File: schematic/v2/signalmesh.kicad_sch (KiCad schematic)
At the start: 164 parts, among them J1 FPGA I/O, J10 INA219_CONFIG, J11 INA219_CONFIG, J12 AAM_DBG, J13 UUM_DBG, J14 ACM_DBG, J15 INA219_CONFIG, J16 DSM_DBG, J17 LCD_display, J18 LCD_display, J19 AudioJack3, J2 FPGA I/O, J20 USB3_A, J21 USB_A, J23 USB_A, J3 LCD_display, J4 TDM_DBG, J5 INA219_CONFIG, J6 INA219_CONFIG, J7 INA219_CONFIG, J8 FPGA I/O, J9 FPGA I/O, U1 NUCLEO-H753ZI, U10 INA219AxD, U11 INA219AxD, U12 INA219AxD, U13 INA219AxD, U14 W25Q128JVS, U15 AP2112K-3.3, U16 74HC4050D, U17 NUCLEO-H753ZI, U18 HDSP-7503, U19 HDSP-7503, U2 HDSP-7503, U20 INA219AxD, U21 74HC4050D, U22 AP2112K-3.3, U23 W25Q128JVS, U24 74HC4050D, U25 AP2112K-3.3, U26 W25Q128JVS, U27 MCP2551-I-P, U28 74LVC1G3157, U29 MCP2551-I-P, U3 NUCLEO-F303RE, U30 MCP2551-I-P, U31 MCP2551-I-P, U32 CH340G, U4 YAAJ_BluePill_Part_Like, U5 24LC256-I_SN, U6 BME280, U7 INA219AxD, U8 24LC256-I_SN, U9 NUCLEO-F446RE, Y1 Crystal

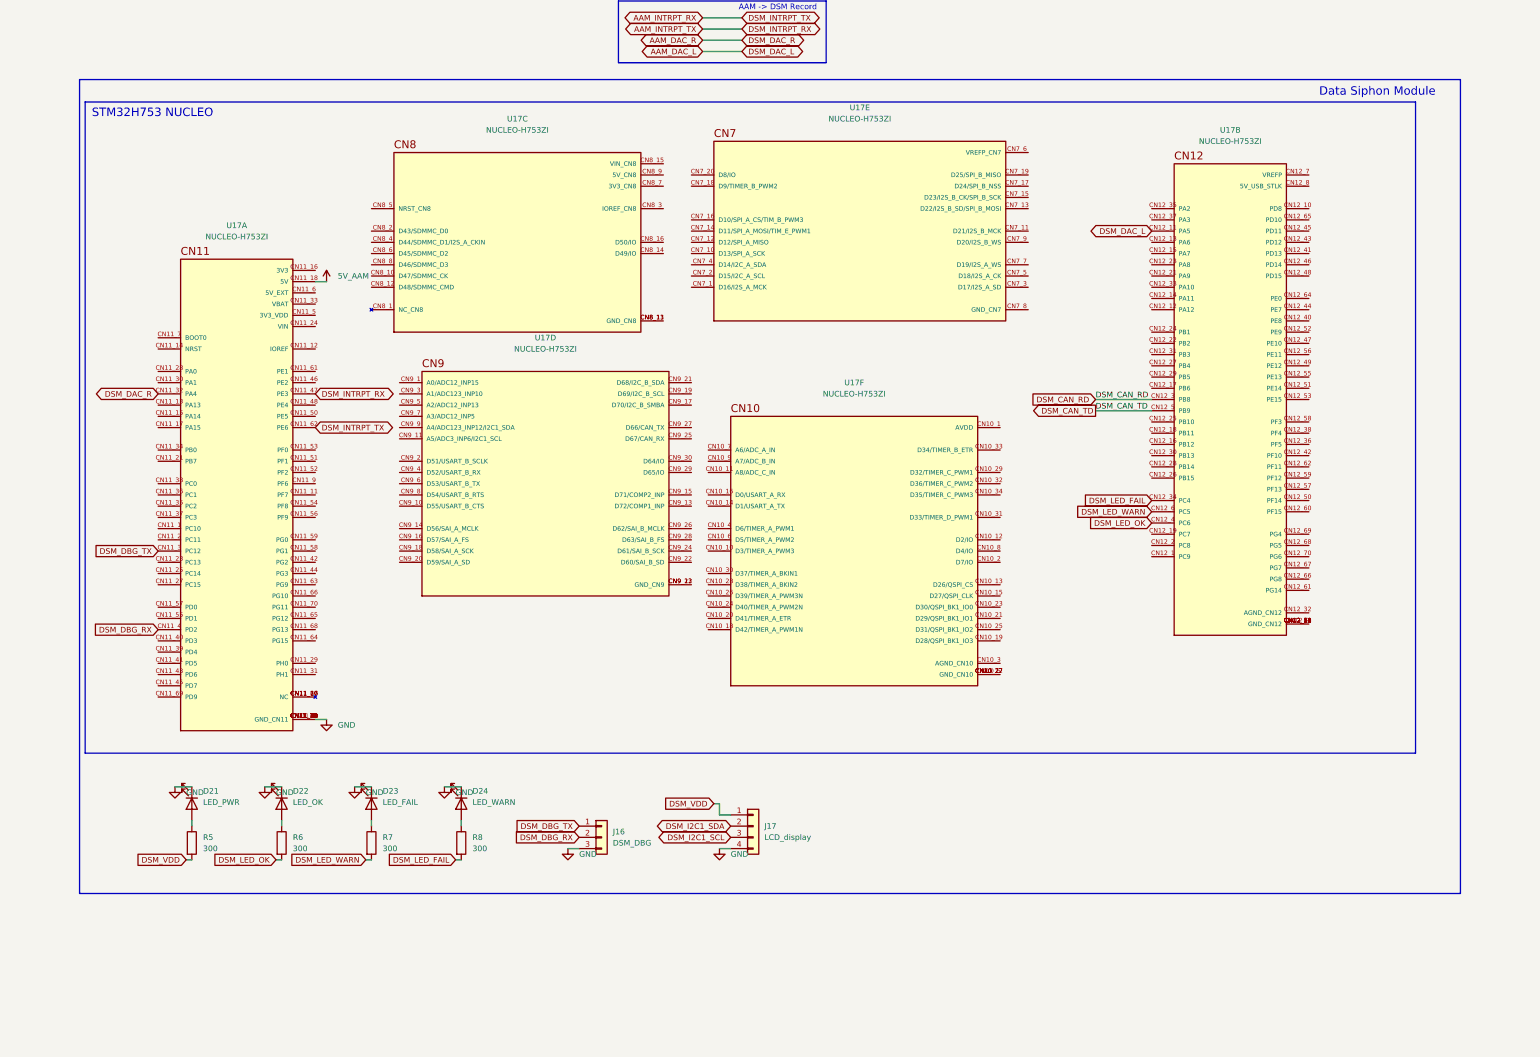
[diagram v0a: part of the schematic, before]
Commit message: i should really make this multiple sheets
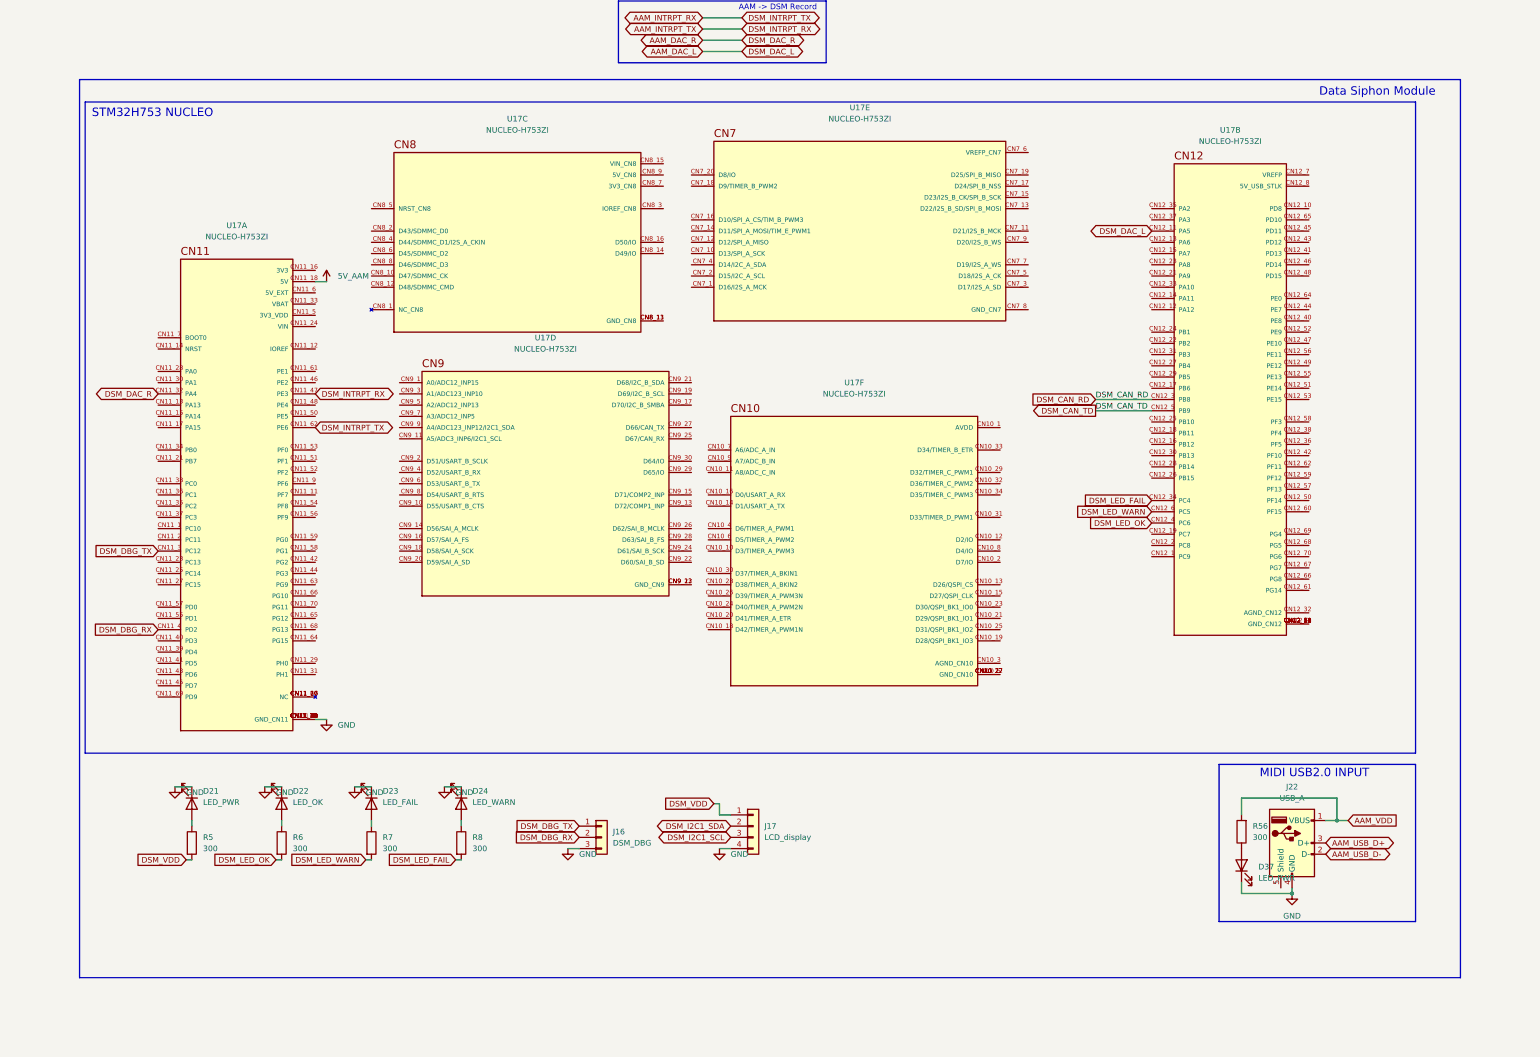
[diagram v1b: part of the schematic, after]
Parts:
- added D37: LED_PWR, LED_SMD:LED_0603_1608Metric, symbol Device:LED
- added J22: USB_A, Connector_USB:USB_A_CNCTech_1001-011-01101_Horizontal, symbol Connector:USB_A
- added R56: 300, Resistor_SMD:R_0805_2012Metric_Pad1.20x1.40mm_HandSolder, symbol Device:R
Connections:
- net AAM_USB_D+: now also J22.3 (D+)
- net AAM_USB_D-: now also J22.2 (D-)
- net AAM_VDD: now also J22.1 (VBUS), R56.2
- net GND: now also D37.1 (K), J22.4 (GND)
- new net: D37.2 (A), R56.1
